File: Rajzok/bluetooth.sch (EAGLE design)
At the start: 17 parts, among them Q1 TP0602N2, Q2 TP0602N2, Q3 SUP75N06-08, Q4 SUP75N06-08

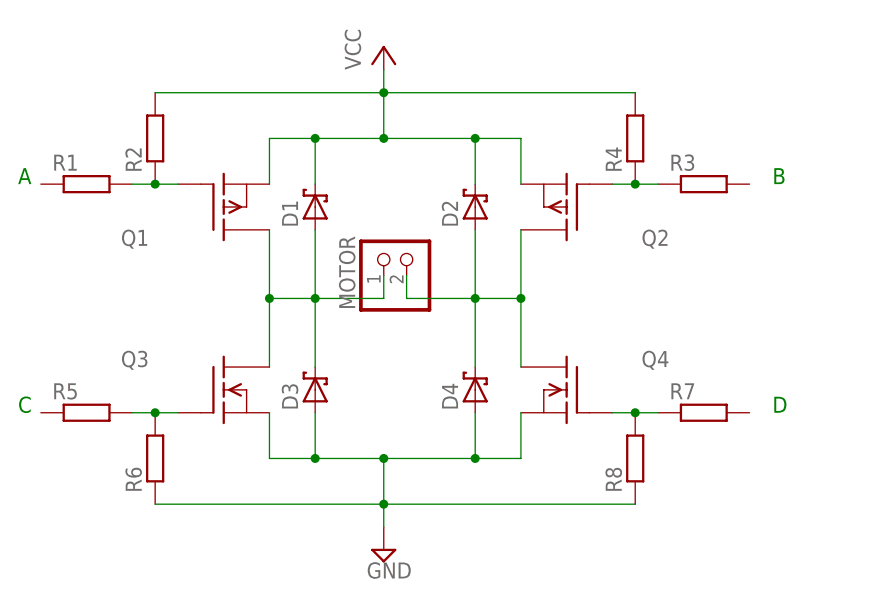
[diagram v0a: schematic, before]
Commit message: Rajzok 2017
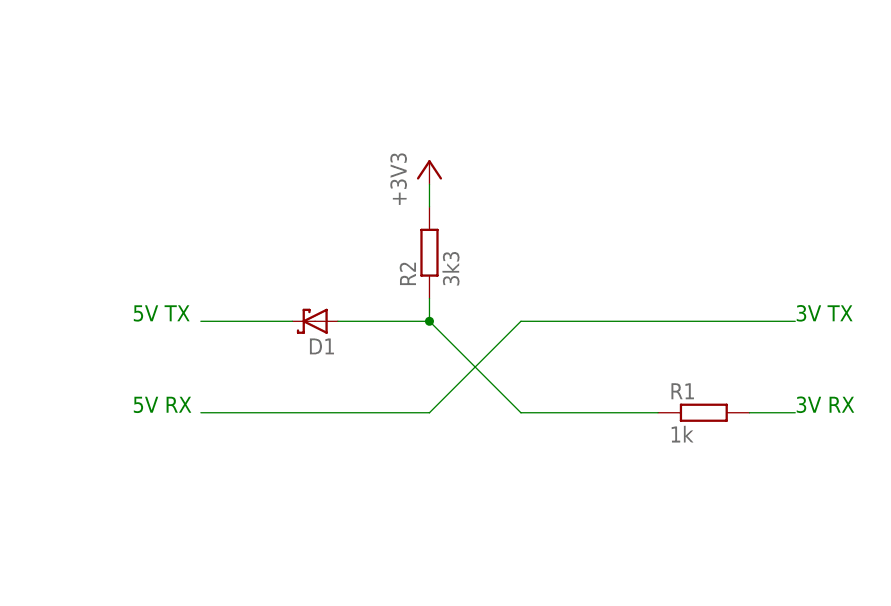
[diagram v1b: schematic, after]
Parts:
- removed D2, D3, D4: 1N6267A, diode:1N6267A
- removed MOTOR: (no value), pinhead:PINHD-1X2
- removed Q1, Q2: TP0602N2, transistor-fet:TP0602N2
- removed Q3, Q4: SUP75N06-08, transistor-fet:SUP75N06-08
- removed R3, R4, R5, R6, R7, R8: (no value), rcl:R-EU_0204/7
- D1: value 1N6267A -> (none); device diode:1N6267A -> diode:SCHOTTKY-DIODEF126Z12
- R1: value (none) -> 1k; device rcl:R-EU_0204/7 -> rcl:R-EU_0207/5V
- R2: value (none) -> 3k3; device rcl:R-EU_0204/7 -> rcl:R-EU_0207/5V
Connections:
- removed net GND: D3.A, D4.A, Q3.S, Q4.S, R6.1, R8.1
- removed net N$3: Q2.G, R3.1, R4.1
- removed net N$5: Q4.G, R7.1, R8.2
- removed net N$9: D1.A, D3.C, MOTOR.1, Q1.D, Q3.D
- removed net VCC: D1.C, D2.C, Q1.S, Q2.S, R2.2, R4.2
- new net +3V3: R2.2
- net N$1: now also D1.A, R1.1; no longer Q1.G, R1.2
- net N$2: now also R1.2; no longer D2.A, D4.C, MOTOR.2, Q2.D, Q4.D
- net N$4: now also D1.C; no longer Q3.G, R5.2, R6.2
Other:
- note added: "3V RX"
- note added: "3V TX"
- note added: "5V RX"
- note added: "5V TX"
- note removed: "A"
- note removed: "B"
- note removed: "C"
- note removed: "D"
- moved on the sheet: R1, R2
